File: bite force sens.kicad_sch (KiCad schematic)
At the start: 19 parts, among them J1 Flexiforce, J2 oled display, J4 switch, J6 Conn_01x02, J7 Conn_01x02, U1 XIAO ESP32 S3, U2 MCP6004

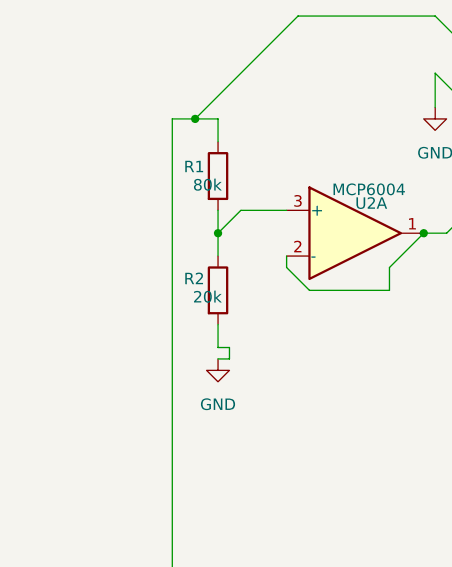
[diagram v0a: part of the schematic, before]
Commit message: added ressitor
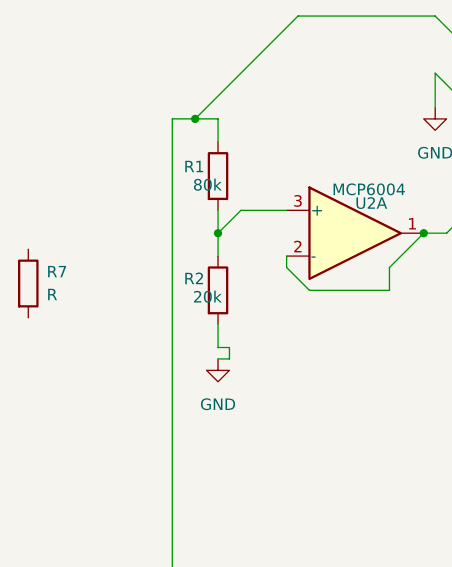
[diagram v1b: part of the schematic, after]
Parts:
- added R7: R, symbol Device:R
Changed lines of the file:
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@@
+	)
+	(symbol
+		(lib_id "Device:R")
+		(at 89.408 107.188 0)
+		(unit 1)
+		(exclude_from_sim no)
+		(in_bom yes)
+		(on_board yes)
+		(dnp no)
+		(fields_autoplaced yes)
+		(property "Reference" "R7"
+			(at 91.44 105.9179 0)
+			(effects
+				(font
+					(size 1.27 1.27)
+				)
+				(justify left)
+			)
+		)
+		(property "Value" "R"
+			(at 91.44 108.4579 0)
+			(effects
+				(font
+					(size 1.27 1.27)
+				)
+				(justify left)
+			)
+		)
+		(property "Footprint" ""
+			(at 87.63 107.188 90)
+			(effects
+				(font
+					(size 1.27 1.27)
+				)
+				(hide yes)
+			)
+		)
+		(property "Datasheet" "~"
+			(at 89.408 107.188 0)
+			(effects
+				(font
+					(size 1.27 1.27)
+				)
+				(hide yes)
+			)
+		)
+		(property "Description" "Resistor"
+			(at 89.408 107.188 0)
+			(effects
+				(font
+					(size 1.27 1.27)
+				)
+				(hide yes)
+			)
+		)
+		(pin "1"
+		)
+		(pin "2"
+		)
+		(instances
+			(project ""
+				(path "/3593a1b8-1220-470f-a3ee-4529e20730d6"
+					(reference "R7")
+					(unit 1)
+				)
+			)
+		)
 	)
 	(symbol

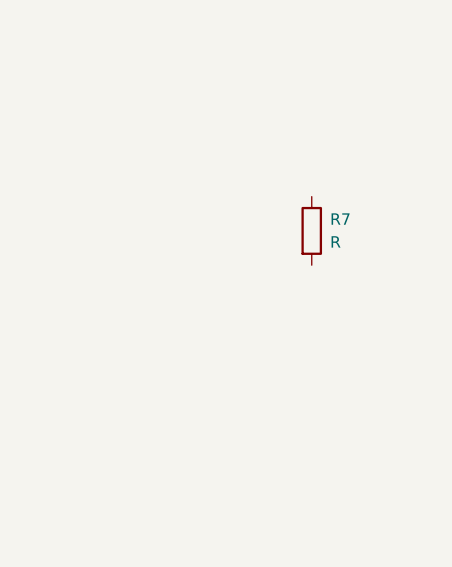
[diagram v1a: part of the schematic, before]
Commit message: added ressitor again
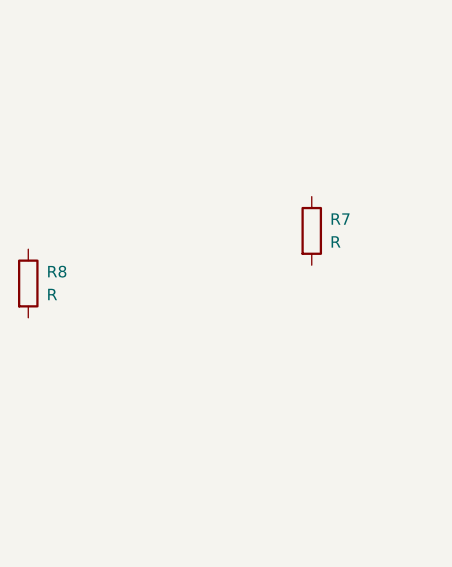
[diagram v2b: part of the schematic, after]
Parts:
- added R8: R, symbol Device:R
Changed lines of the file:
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@@
+	(symbol
+		(lib_id "Device:R")
+		(at 57.912 113.03 0)
+		(unit 1)
+		(exclude_from_sim no)
+		(in_bom yes)
+		(on_board yes)
+		(dnp no)
+		(fields_autoplaced yes)
+		(property "Reference" "R8"
+			(at 59.944 111.7599 0)
+			(effects
+				(font
+					(size 1.27 1.27)
+				)
+				(justify left)
+			)
+		)
+		(property "Value" "R"
+			(at 59.944 114.2999 0)
+			(effects
+				(font
+					(size 1.27 1.27)
+				)
+				(justify left)
+			)
+		)
+		(property "Footprint" ""
+			(at 56.134 113.03 90)
+			(effects
+				(font
+					(size 1.27 1.27)
+				)
+				(hide yes)
+			)
+		)
+		(property "Datasheet" "~"
+			(at 57.912 113.03 0)
+			(effects
+				(font
+					(size 1.27 1.27)
+				)
+				(hide yes)
+			)
+		)
+		(property "Description" "Resistor"
+			(at 57.912 113.03 0)
+			(effects
+				(font
+					(size 1.27 1.27)
+				)
+				(hide yes)
+			)
+		)
+		(pin "1"
+		)
+		(pin "2"
+		)
+		(instances
+			(project "bite force sens"
+				(path "/3593a1b8-1220-470f-a3ee-4529e20730d6"
+					(reference "R8")
+					(unit 1)
+				)
+			)
+		)
+	)
 	(symbol
 		(lib_id "Device:R")

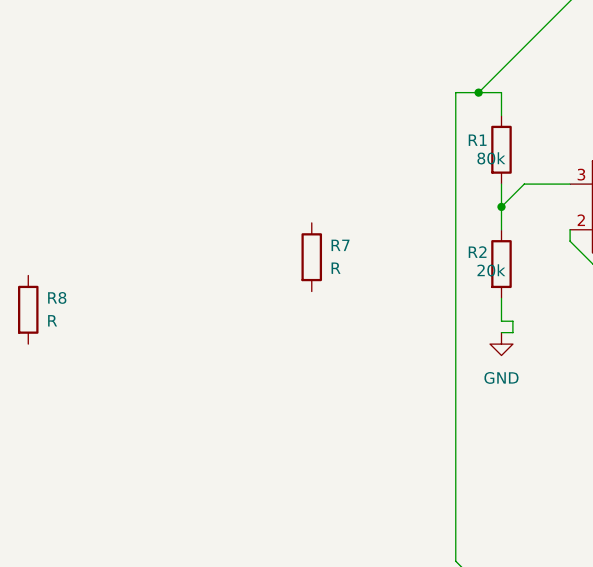
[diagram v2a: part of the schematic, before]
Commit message: removed un
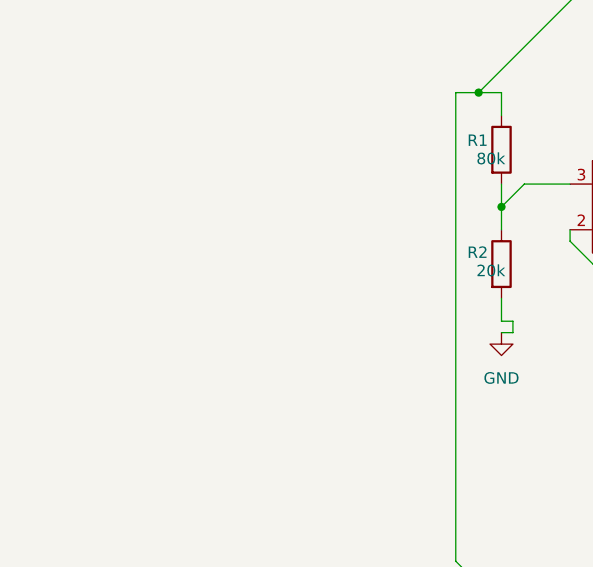
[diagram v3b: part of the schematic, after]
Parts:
- removed R7, R8: R, symbol Device:R
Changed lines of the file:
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@@
-	(symbol
-		(lib_id "Device:R")
-		(at 57.912 113.03 0)
-		(unit 1)
-		(exclude_from_sim no)
-		(in_bom yes)
-		(on_board yes)
-		(dnp no)
-		(fields_autoplaced yes)
-		(property "Reference" "R8"
-			(at 59.944 111.7599 0)
-			(effects
-				(font
-					(size 1.27 1.27)
-				)
-				(justify left)
-			)
-		)
-		(property "Value" "R"
-			(at 59.944 114.2999 0)
-			(effects
-				(font
-					(size 1.27 1.27)
-				)
-				(justify left)
-			)
-		)
-		(property "Footprint" ""
-			(at 56.134 113.03 90)
-			(effects
-				(font
-					(size 1.27 1.27)
-				)
-				(hide yes)
-			)
-		)
-		(property "Datasheet" "~"
-			(at 57.912 113.03 0)
-			(effects
-				(font
-					(size 1.27 1.27)
-				)
-				(hide yes)
-			)
-		)
-		(property "Description" "Resistor"
-			(at 57.912 113.03 0)
-			(effects
-				(font
-					(size 1.27 1.27)
-				)
-				(hide yes)
-			)
-		)
-		(pin "1"
-		)
-		(pin "2"
-		)
-		(instances
-			(project "bite force sens"
-				(path "/3593a1b8-1220-470f-a3ee-4529e20730d6"
-					(reference "R8")
-					(unit 1)
-				)
-			)
-		)
-	)
 	(symbol
 		(lib_id "Device:R")
@@
 					(unit 1)
 				)
-			)
-		)
-	)
-	(symbol
-		(lib_id "Device:R")
-		(at 89.408 107.188 0)
-		(unit 1)
-		(exclude_from_sim no)
-		(in_bom yes)
-		(on_board yes)
-		(dnp no)
-		(fields_autoplaced yes)
-		(property "Reference" "R7"
-			(at 91.44 105.9179 0)
-			(effects
-				(font
-					(size 1.27 1.27)
-				)
-				(justify left)
-			)
-		)
-		(property "Value" "R"
-			(at 91.44 108.4579 0)
-			(effects
-				(font
-					(size 1.27 1.27)
-				)
-				(justify left)
-			)
-		)
-		(property "Footprint" ""
-			(at 87.63 107.188 90)
-			(effects
-				(font
-					(size 1.27 1.27)
-				)
-				(hide yes)
-			)
-		)
-		(property "Datasheet" "~"
-			(at 89.408 107.188 0)
-			(effects
-				(font
-					(size 1.27 1.27)
-				)
-				(hide yes)
-			)
-		)
-		(property "Description" "Resistor"
-			(at 89.408 107.188 0)
-			(effects
-				(font
-					(size 1.27 1.27)
-				)
-				(hide yes)
-			)
-		)
-		(pin "1"
-		)
-		(pin "2"
-		)
-		(instances
-			(project ""
-				(path "/3593a1b8-1220-470f-a3ee-4529e20730d6"
-					(reference "R7")
-					(unit 1)
-				)
